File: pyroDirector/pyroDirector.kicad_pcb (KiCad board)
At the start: 4 copper layers, 100 x 100 mm, 93 parts, among them J1 Conn_01x03_Male, J10 BTNS, J11 DC_Conv, J12 CALIB_MODULE, J13 DISP_I2C, J14 Conn_01x03_Male, J15 SJ1-2503A, J16 Conn_01x03_Male, J17 SJ1-2503A, J18 Conn_01x03_Male, J19 SJ1-2503A, J2 AudioJack3.5mm, J20 LED_ext, J21 Screw_Terminal_01x02, J22 LED_ext, J23 Screw_Terminal_01x02, J24 LED_ext, J25 Screw_Terminal_01x02, J3 Header_A1-A15, J4 Header_D14-19, J5 Header_D48-53, J6 V_Batt, J7 Header_ISP, J8 PWR_SWITCH, J9 Batt, K1 PR12-5V-360-1C, K2 PR12-5V-360-1C, K3 PR12-5V-360-1C, Q1 MMBT2222A 1P, Q10 MMBT2222A 1P, Q11 IRLB8721PbF, Q12 MMBT2222A 1P, Q13 IRLB8721PbF, Q2 MMBT2222A 1P, Q3 MMBT2222A 1P, Q4 MMBT2222A 1P, Q5 MMBT2222A 1P, Q6 MMBT2222A 1P, Q7 MMBT2222A 1P, Q8 MMBT2222A 1P, Q9 IRLB8721PbF, SW1 SW_Enable, U1 MEGA_PRO_ATMEGA2560

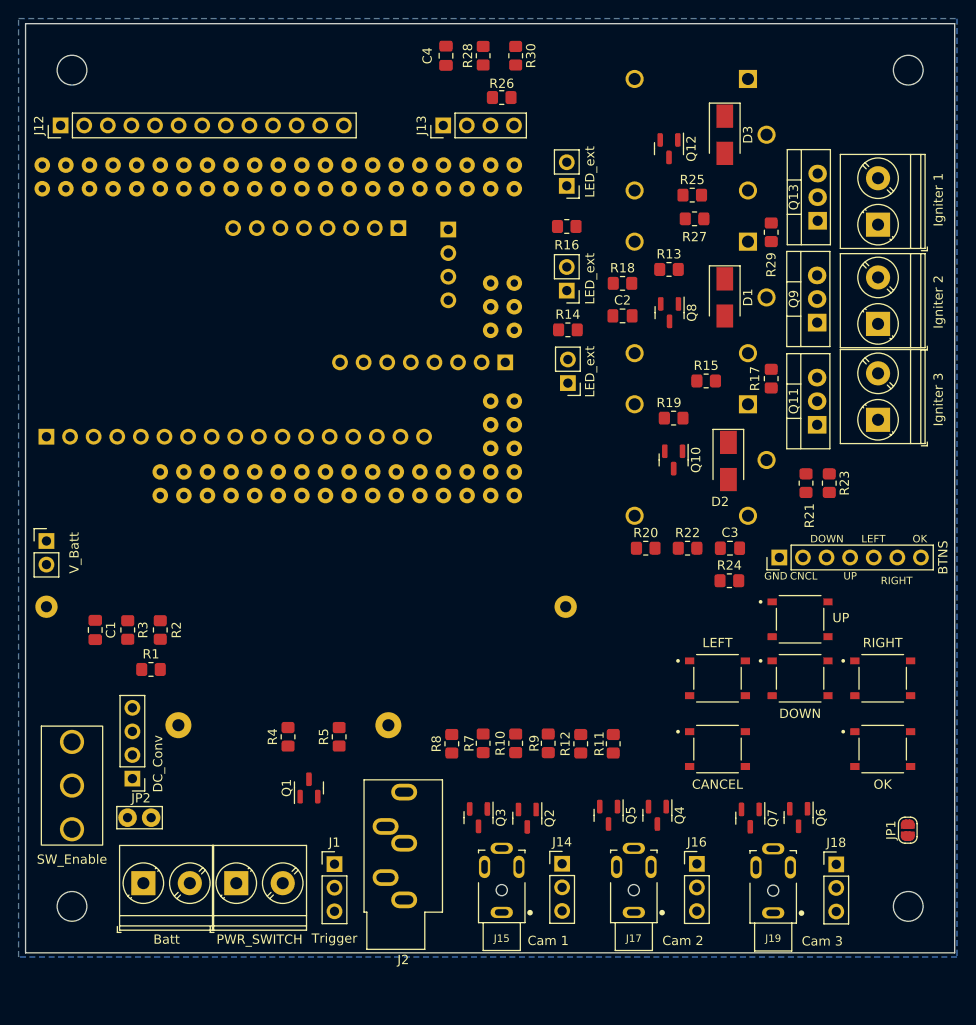
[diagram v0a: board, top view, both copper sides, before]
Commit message: placement & 3-D models complete
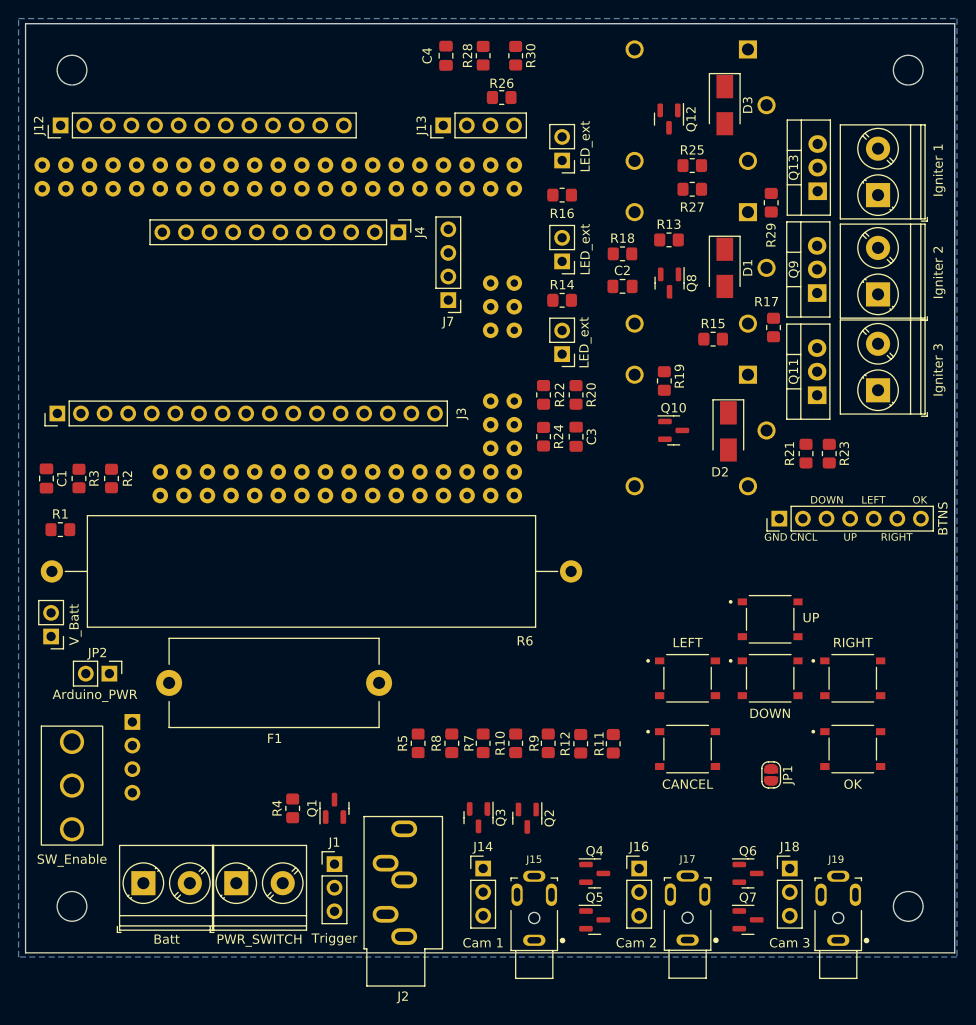
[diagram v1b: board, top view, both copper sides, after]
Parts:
- removed J5: Header_D48-53, Connector_PinHeader_2.54mm:PinHeader_1x08_P2.54mm_Vertical
- F1, J3, J7, R6: moved to F.Cu
- J11: moved to B.Cu
- J4: value Header_D14-19 -> Header_D14-19_D49_51_53; footprint Connector_PinHeader_2.54mm:PinHeader_1x08_P2.54mm_Vertical -> Connector_PinHeader_2.54mm:PinHeader_1x11_P2.54mm_Vertical; moved to F.Cu
- JP2: footprint TestPoint:TestPoint_Bridge_Pitch2.54mm_Drill1.0mm -> Connector_PinHeader_2.54mm:PinHeader_1x02_P2.54mm_Vertical
- moved R24 25.3 mm to (152.5, 87.0), turned to -90 degrees
- moved R22 22.6 mm to (152.5, 82.5), turned to 90 degrees
- moved C3 20.5 mm to (156.0, 87.0), turned to -90 degrees
- moved R20 18.1 mm to (156.0, 82.5), turned to -90 degrees
- moved R1 17.9 mm to (100.5, 97.0)
- moved C1 17.1 mm to (99.0, 91.5)
- moved R2 17.1 mm to (106.0, 91.5)
- moved R3 17.1 mm to (102.5, 91.5)
- moved JP2 16.1 mm to (105.8, 112.5), turned to -90 degrees
- moved JP1 15.9 mm to (177.0, 123.4), turned to -90 degrees
- moved Q5 11.3 mm to (158.0, 139.0), turned to 0 degrees
- moved Q7 11.0 mm to (174.5, 139.0), turned to 0 degrees
- moved J6 10.3 mm to (99.5, 108.5), turned to 180 degrees
- moved Q4 9.20 mm to (158.0, 134.0), turned to 0 degrees
- moved R5 8.53 mm to (139.0, 120.0)
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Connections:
- J4 pad 2: /D19 -> /D53
- J4 pad 3: /D18 -> /D51
- J4 pad 4: /D17 -> /D49
- J4 pad 5: /D16 -> /D19
- J4 pad 6: /D15 -> /D18
- J4 pad 7: /D14 -> /D17
- J4 pad 8: GND -> /D16
- JP2 pad 1: +5V -> /VO+
- U1 pad D26: /FIRE_1 -> unconnected-(U1-PadD26)
- U1 pad D28: /PRIME_2 -> unconnected-(U1-PadD28)
- U1 pad D30: /SENSE_2 -> unconnected-(U1-PadD30)
- U1 pad D32: /BTN_OK -> /TRIGGER_LED
- U1 pad D33: /BTN_UP -> /TRIGGER
- U1 pad D34: /BTN_DOWN -> /PRE_CAM_0
- U1 pad D35: /BTN_RIGHT -> /SHUTTER_CAM_0
- U1 pad D36: /BTN_LEFT -> /PRE_CAM_1
- U1 pad D37: /BTN_CNCL -> /SHUTTER_CAM_1
- U1 pad D38: /TRIGGER_LED -> /PRE_CAM_2
- U1 pad D39: /TRIGGER -> /SHUTTER_CAM_2
- U1 pad D40: unconnected-(U1-PadD40) -> /BTN_OK
- U1 pad D41: unconnected-(U1-PadD41) -> /BTN_UP
- U1 pad D42: /PRE_CAM_0 -> /BTN_DOWN
- U1 pad D43: /SHUTTER_CAM_0 -> /BTN_RIGHT
- U1 pad D44: /PRE_CAM_1 -> /BTN_LEFT
- U1 pad D45: /SHUTTER_CAM_1 -> /BTN_CNCL
- U1 pad D46: /PRE_CAM_2 -> unconnected-(U1-PadD46)
- U1 pad D47: /SHUTTER_CAM_2 -> unconnected-(U1-PadD47)
- U1 pad D48: /D48 -> /SENSE_2
- U1 pad D50: /D50 -> /PRIME_2
- U1 pad D52: /D52 -> /FIRE_1
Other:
- board text added: "EN"
- board text added: "Vin+"
- board text added: "Vo+"
